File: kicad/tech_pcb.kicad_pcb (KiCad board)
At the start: 2 copper layers, 18.3 x 31.7 mm, 24 parts, among them J1 Conn_01x10, J2 Conn_01x10, J3 USB_C_Receptacle_USB2.0_16P, J4 Conn_01x03_MountingPin, SW1 SW_Push, SW2 SW_Push, U1 STM32C071GBUxN, U2 XC6206PxxxMR

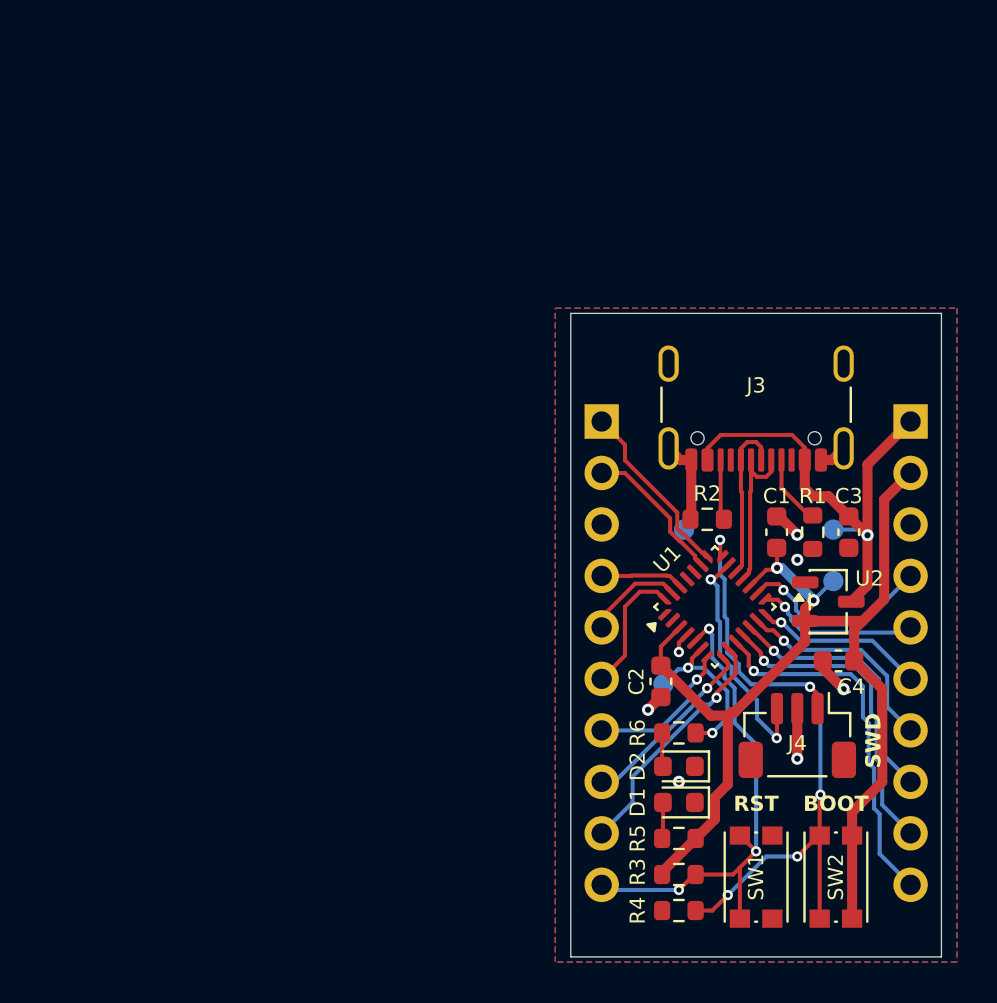
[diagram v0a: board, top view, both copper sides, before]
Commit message: Update board to v0.2
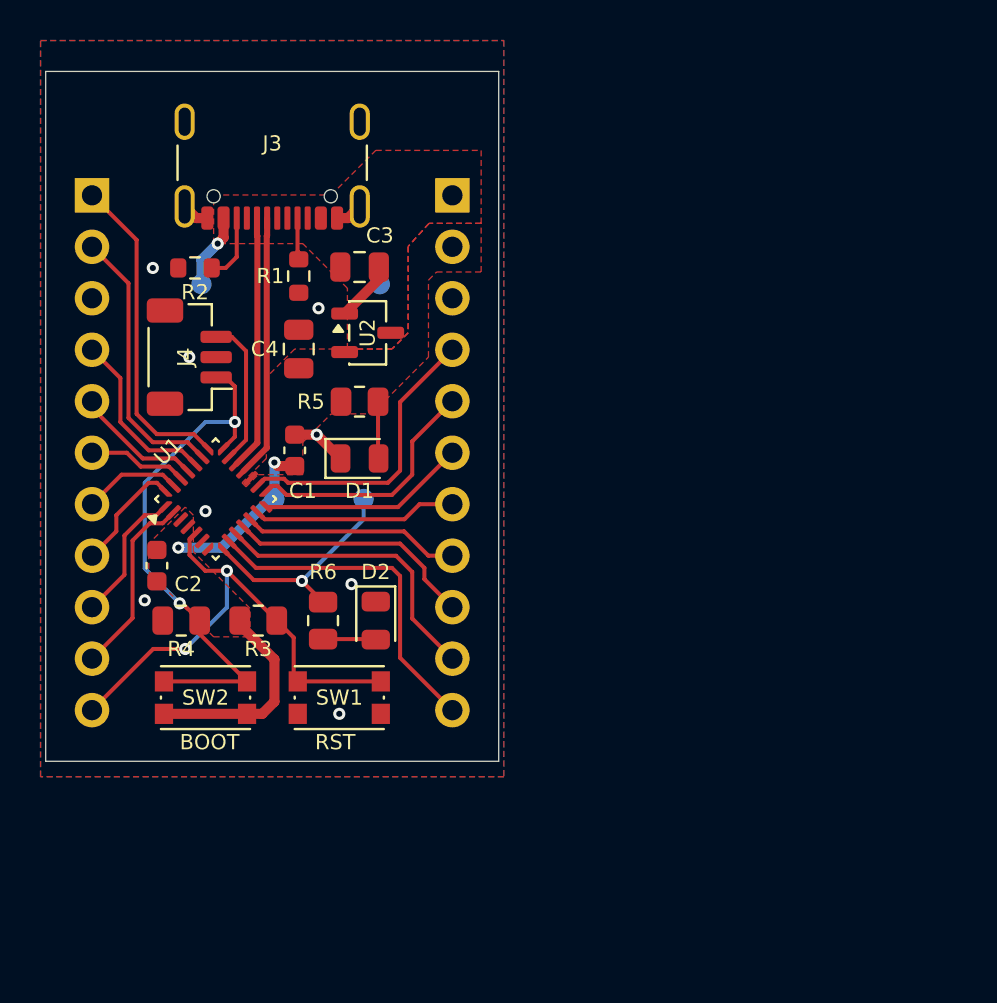
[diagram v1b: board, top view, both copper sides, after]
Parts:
- C3, C4: footprint Capacitor_SMD:C_0603_1608Metric -> Capacitor_SMD:C_0805_2012Metric
- D1, D2: footprint LED_SMD:LED_0603_1608Metric -> LED_SMD:LED_0805_2012Metric
- J1, J2: value Conn_01x10 -> Conn_01x11; footprint Connector_PinHeader_2.54mm:PinHeader_1x10_P2.54mm_Vertical -> Connector_PinHeader_2.54mm:PinHeader_1x11_P2.54mm_Vertical
- R3, R4, R5, R6: footprint Resistor_SMD:R_0603_1608Metric -> Resistor_SMD:R_0805_2012Metric
- SW1: value SW_Push -> RST
- SW2: value SW_Push -> BOOT
- moved J4 35.3 mm to (30.2, 33.4), turned to 90 degrees
- moved TP3 33.4 mm to (30.8, 29.8)
- moved SW2 32.3 mm to (31.0, 50.2), turned to 0 degrees
- moved C4 30.8 mm to (35.6, 33.0), turned to 90 degrees
- moved R4 28.4 mm to (29.8, 46.4)
- moved R1 28.3 mm to (35.6, 29.4)
- moved R2 28.2 mm to (30.5, 29.0)
- moved TP1 27.9 mm to (34.4, 40.4)
- moved J1 27.5 mm to (25.4, 25.4)
- moved C3 27.5 mm to (38.6, 29.0), turned to 0 degrees
- moved R5 26.7 mm to (38.6, 35.6), turned to 0 degrees
- moved J3 26.7 mm to (34.3, 22.9)
- moved U2 26.3 mm to (39.0, 32.2)
- moved C2 25.5 mm to (28.6, 43.7)
- moved J2 25.2 mm to (43.2, 25.4)
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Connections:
- J1 pad 10: /NRST -> /PC14
- J1 pad 4: /PB6 -> /PB4
- J1 pad 5: /PB7 -> /PB5
- J1 pad 6: /PB8 -> /PB6
- J1 pad 7: /PA1 -> /PB7
- J1 pad 8: /PA2 -> /PB8
- J1 pad 9: /PA3 -> /PC15
- U1 pad 1: unconnected-(U1-PC14-Pad1) -> /PC15
- U1 pad 2: unconnected-(U1-PC15-Pad2) -> /PC14
- U1 pad 24: unconnected-(U1-PB4-Pad24) -> /PB4
- U1 pad 25: unconnected-(U1-PB5-Pad25) -> /PB5
- U1 pad 6: /STATUS -> unconnected-(U1-PA0-Pad6)
- U1 pad 7: /PA1 -> unconnected-(U1-PA1-Pad7)
- U1 pad 8: /PA2 -> /STATUS
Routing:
- net +3V3: track 57.4 -> 18.7 mm
- net +5V: track 23.9 -> 3.71 mm
- net /PA2: track 9.30 -> 0.00 mm, vias 1 -> 0
- net /PC14: track 0.00 -> 9.25 mm
- net /PB4: track 0.00 -> 8.69 mm
- net /PA1: track 7.44 -> 0.00 mm, vias 1 -> 0
- net /PA15: track 8.92 -> 16.0 mm
- net /PC15: track 0.00 -> 6.83 mm
- net /PB3: track 7.26 -> 13.6 mm
- net /PB5: track 0.00 -> 6.35 mm
- net /BOOT0: track 32.1 -> 26.2 mm, vias 5 -> 2
- net GND: track 13.4 -> 8.46 mm, vias 7 -> 8
- net /PA3: track 12.1 -> 16.8 mm, vias 1 -> 0
- net /USB_DP: track 7.96 -> 12.6 mm
- net /PA8: track 9.97 -> 14.5 mm, vias 1 -> 0
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- added copper zone on F.Cu, net +3V3
- added copper zone on F.Cu, net +5V
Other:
- board size 18.3 x 31.7 mm -> 22.4 x 34 mm
- board text added: "TN Tech PCB Workshop Prototype v0.2"
- board text removed: "SWD"
- board text removed: "TTU PCB Workshop Prototype v0.1"
